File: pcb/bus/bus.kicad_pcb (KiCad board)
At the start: 4 copper layers, 170 x 55 mm, 0 parts

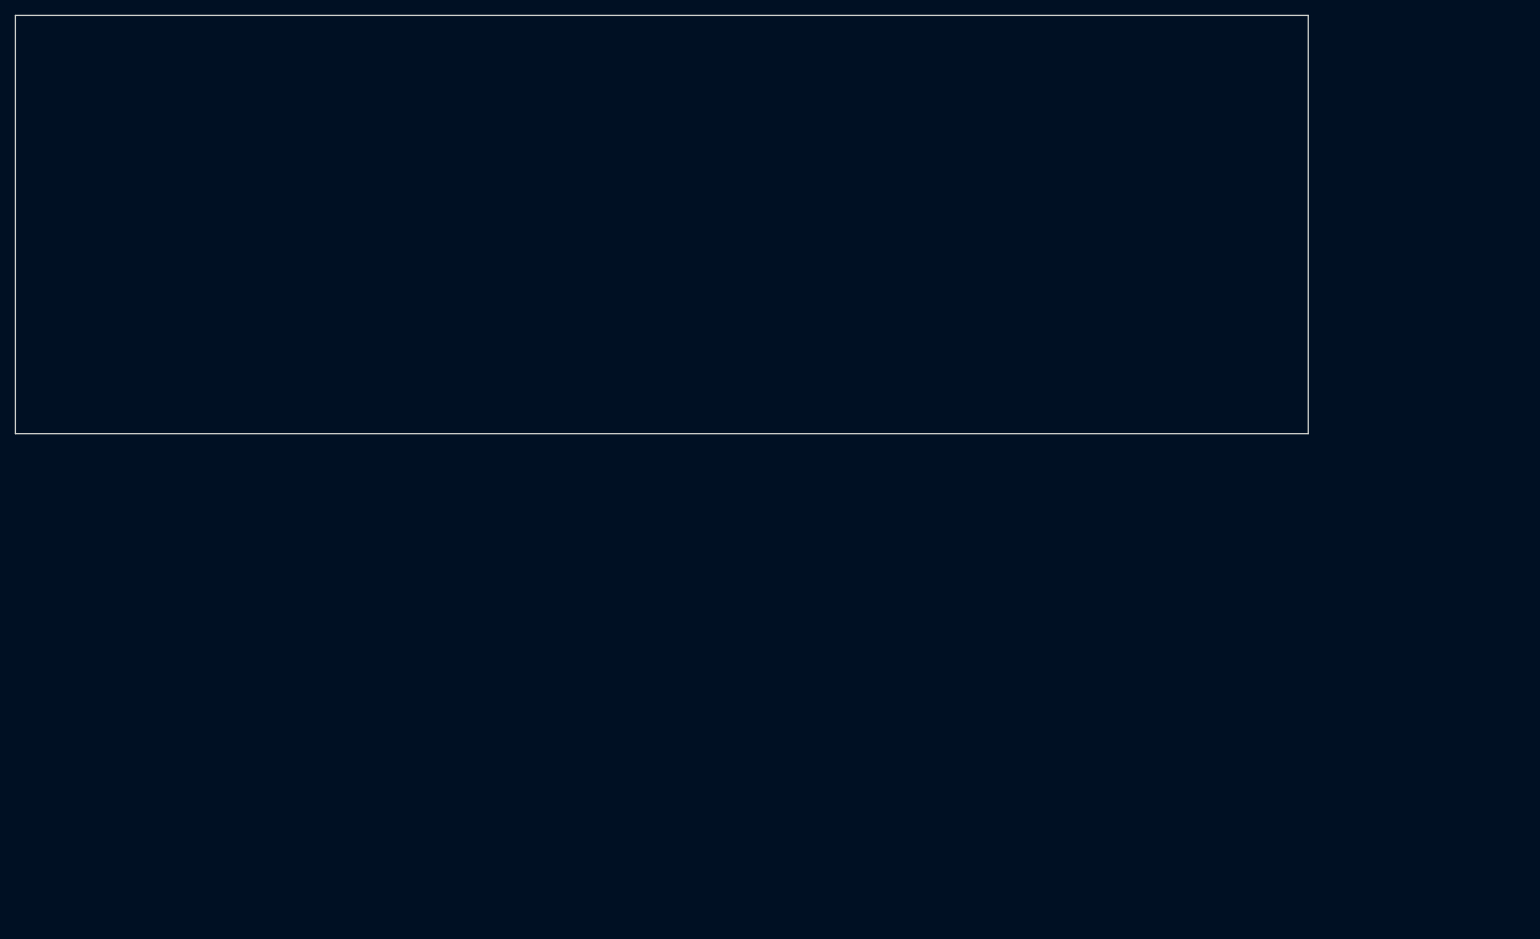
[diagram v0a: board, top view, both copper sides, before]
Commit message: update bus pcb
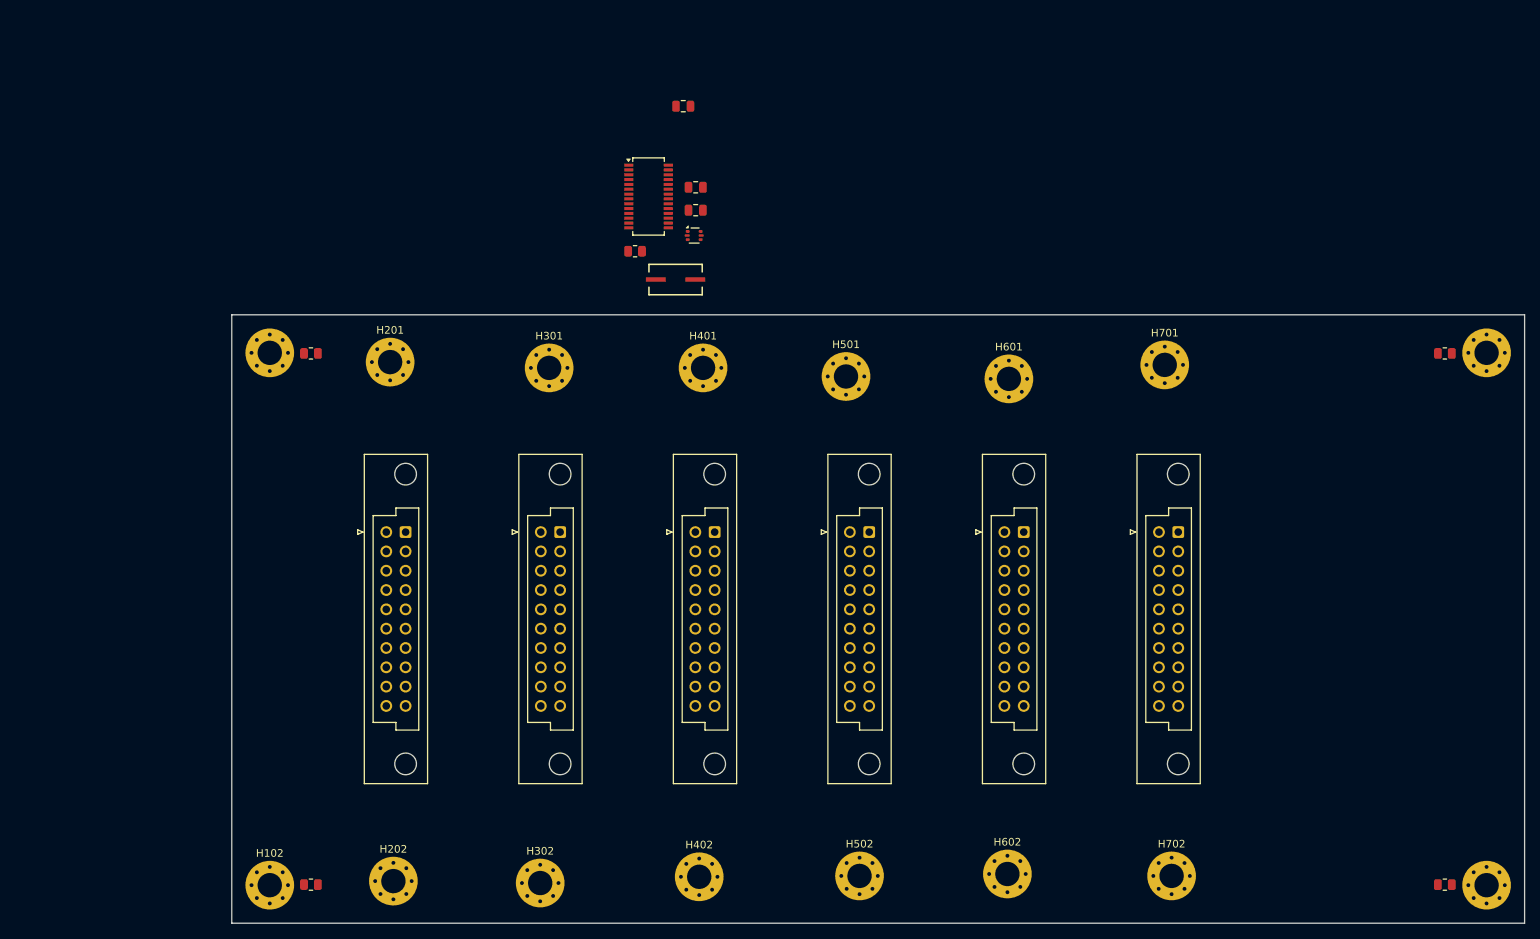
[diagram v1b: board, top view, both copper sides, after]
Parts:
- added C101: 10uF, Capacitor_SMD:C_0805_2012Metric, F.Cu at (114.2, 33.4)
- added C102: 10uF, Capacitor_SMD:C_0805_2012Metric, F.Cu at (115.8, 44.1)
- added C103: 100nF, Capacitor_SMD:C_0805_2012Metric, F.Cu at (115.8, 47.1)
- added H101: MountingHole_Pad, MountingHole:MountingHole_3.2mm_M3_Pad_Via, F.Cu at (59.8, 65.8)
- added H102: MountingHole_Pad, MountingHole:MountingHole_3.2mm_M3_Pad_Via, F.Cu at (59.8, 135.8)
- added H103: MountingHole_Pad, MountingHole:MountingHole_3.2mm_M3_Pad_Via, F.Cu at (219.8, 135.8)
- added H104: MountingHole_Pad, MountingHole:MountingHole_3.2mm_M3_Pad_Via, F.Cu at (219.8, 65.8)
- added H201: MountingHole_Pad, MountingHole:MountingHole_3.2mm_M3_Pad_Via, F.Cu at (75.6, 67.0)
- added H202: MountingHole_Pad, MountingHole:MountingHole_3.2mm_M3_Pad_Via, F.Cu at (76.0, 135.3)
- added H301: MountingHole_Pad, MountingHole:MountingHole_3.2mm_M3_Pad_Via, F.Cu at (96.5, 67.8)
- added H302: MountingHole_Pad, MountingHole:MountingHole_3.2mm_M3_Pad_Via, F.Cu at (95.3, 135.5)
- added H401: MountingHole_Pad, MountingHole:MountingHole_3.2mm_M3_Pad_Via, F.Cu at (116.8, 67.8)
- added H402: MountingHole_Pad, MountingHole:MountingHole_3.2mm_M3_Pad_Via, F.Cu at (116.3, 134.7)
- added H501: MountingHole_Pad, MountingHole:MountingHole_3.2mm_M3_Pad_Via, F.Cu at (135.6, 68.9)
- added H502: MountingHole_Pad, MountingHole:MountingHole_3.2mm_M3_Pad_Via, F.Cu at (137.3, 134.6)
- added H601: MountingHole_Pad, MountingHole:MountingHole_3.2mm_M3_Pad_Via, F.Cu at (157.0, 69.2)
- added H602: MountingHole_Pad, MountingHole:MountingHole_3.2mm_M3_Pad_Via, F.Cu at (156.8, 134.4)
- added H701: MountingHole_Pad, MountingHole:MountingHole_3.2mm_M3_Pad_Via, F.Cu at (177.5, 67.4)
- added H702: MountingHole_Pad, MountingHole:MountingHole_3.2mm_M3_Pad_Via, F.Cu at (178.4, 134.6)
- added J201: Conn_02x10_Row_Letter_First, PRJ:PCN10-20P-2.54DSA, F.Cu at (75.1, 89.4)
- added J301: Conn_02x10_Row_Letter_First, PRJ:PCN10-20P-2.54DSA, F.Cu at (95.4, 89.4)
- added J401: Conn_02x10_Row_Letter_First, PRJ:PCN10-20P-2.54DSA, F.Cu at (115.8, 89.4)
- added J501: Conn_02x10_Row_Letter_First, PRJ:PCN10-20P-2.54DSA, F.Cu at (136.1, 89.4)
- added J601: Conn_02x10_Row_Letter_First, PRJ:PCN10-20P-2.54DSA, F.Cu at (156.4, 89.4)
- added J701: Conn_02x10_Row_Letter_First, PRJ:PCN10-20P-2.54DSA, F.Cu at (176.7, 89.4)
- added R101: 2k7, Resistor_SMD:R_0805_2012Metric, F.Cu at (107.8, 52.5)
- added R102: R/C/0Ohm, Resistor_SMD:R_0805_2012Metric, F.Cu at (65.2, 65.9)
- added R103: R/C/0Ohm, Resistor_SMD:R_0805_2012Metric, F.Cu at (65.2, 135.8)
- added R104: R/C/0Ohm, Resistor_SMD:R_0805_2012Metric, F.Cu at (214.3, 135.8)
- added R105: R/C/0Ohm, Resistor_SMD:R_0805_2012Metric, F.Cu at (214.3, 65.9)
- added U101: USBLC6-2SC6, Package_TO_SOT_SMD:SOT-666, F.Cu at (115.6, 50.4)
- added U102: FE1.1s, Package_SO:SSOP-28_3.9x9.9mm_P0.635mm, F.Cu at (109.6, 45.3)
- added Y101: 12MHz, PRJ:M49S-SMD, F.Cu at (113.2, 56.2)
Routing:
- added copper zone on In1.Cu, net GND
- added copper zone on In2.Cu, net GND
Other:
- board size 170 x 55 mm -> 170 x 80 mm
